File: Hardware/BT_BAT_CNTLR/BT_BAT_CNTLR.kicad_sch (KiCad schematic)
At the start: 0 parts

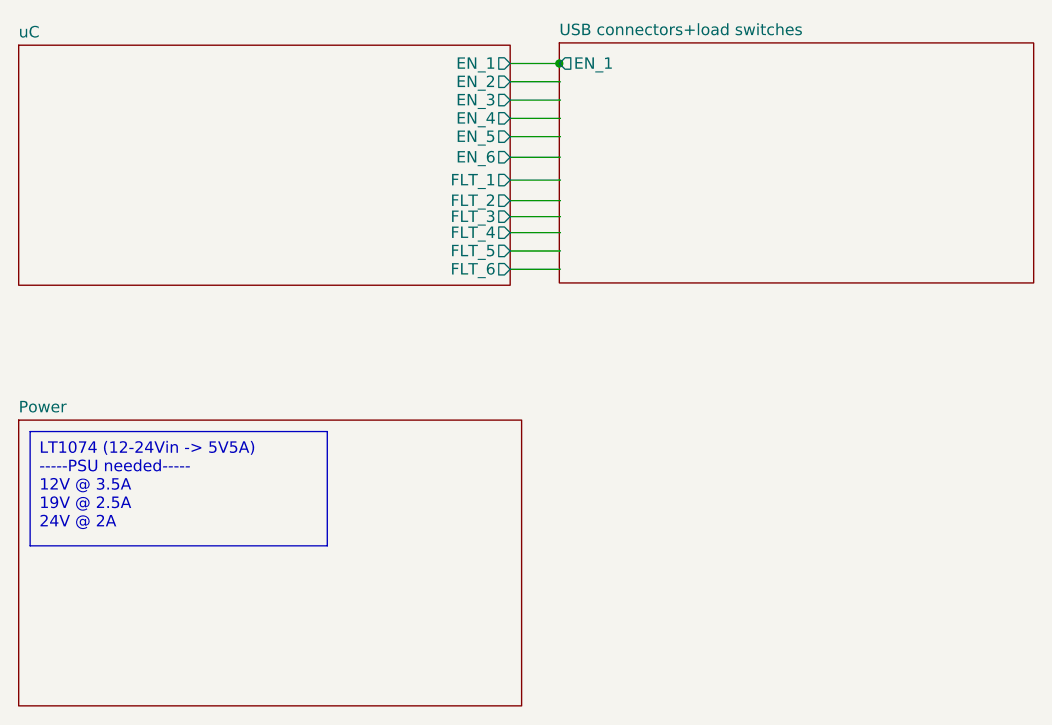
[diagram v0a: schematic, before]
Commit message: - Github Tree Cleanup - Power Routing
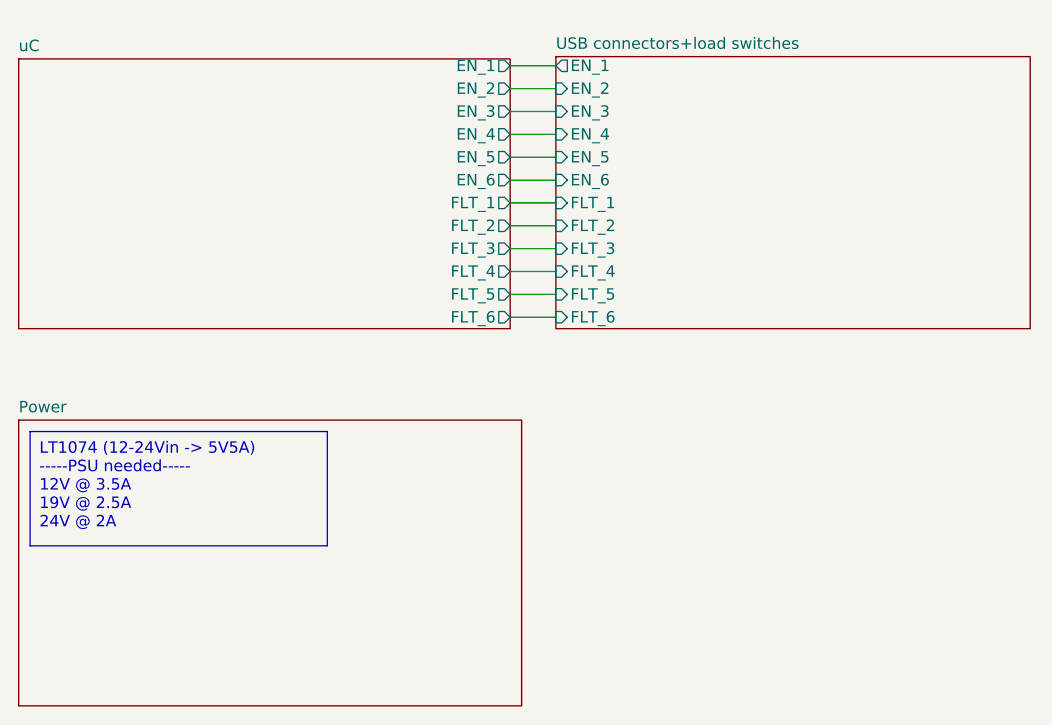
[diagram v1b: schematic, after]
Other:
- sheet USB connectors+load switches ports: added EN_2, EN_3, EN_4, EN_5, EN_6, FLT_1, FLT_2, FLT_3, FLT_4, FLT_5, FLT_6; removed none
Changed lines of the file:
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@@
 (kicad_sch (version 20230121) (generator eeschema)
   (paper "A4")
-  (junction (at 151.511 27.686) (diameter 0) (color 0 0 0 0)
-  )
-  (wire (pts (xy 146.05 38.1) (xy 151.638 38.1))
+  (wire (pts (xy 146.05 35.56) (xy 151.13 35.56))
     (stroke (width 0) (type default))
   )
-  (wire (pts (xy 146.05 29.718) (xy 151.638 29.718))
+  (wire (pts (xy 146.05 30.48) (xy 151.13 30.48))
     (stroke (width 0) (type default))
   )
-  (wire (pts (xy 146.05 27.686) (xy 151.511 27.686))
+  (wire (pts (xy 146.05 45.72) (xy 151.13 45.72))
     (stroke (width 0) (type default))
   )
-  (wire (pts (xy 146.05 33.782) (xy 151.638 33.782))
+  (wire (pts (xy 146.05 50.8) (xy 151.13 50.8))
     (stroke (width 0) (type default))
   )
-  (wire (pts (xy 146.05 46.482) (xy 151.638 46.482))
+  (wire (pts (xy 146.05 33.02) (xy 151.13 33.02))
     (stroke (width 0) (type default))
   )
-  (wire (pts (xy 146.05 42.926) (xy 151.638 42.926))
+  (wire (pts (xy 146.05 27.94) (xy 151.13 27.94))
     (stroke (width 0) (type default))
   )
-  (wire (pts (xy 146.05 50.546) (xy 151.638 50.546))
+  (wire (pts (xy 146.05 55.88) (xy 151.13 55.88))
     (stroke (width 0) (type default))
   )
-  (wire (pts (xy 146.05 48.514) (xy 151.638 48.514))
+  (wire (pts (xy 146.05 38.1) (xy 151.13 38.1))
     (stroke (width 0) (type default))
   )
-  (wire (pts (xy 146.05 40.64) (xy 151.638 40.64))
+  (wire (pts (xy 146.05 43.18) (xy 151.13 43.18))
     (stroke (width 0) (type default))
   )
-  (wire (pts (xy 146.05 35.814) (xy 151.638 35.814))
+  (wire (pts (xy 146.05 53.34) (xy 151.13 53.34))
     (stroke (width 0) (type default))
   )
-  (wire (pts (xy 146.05 44.704) (xy 151.638 44.704))
+  (wire (pts (xy 146.05 40.64) (xy 151.13 40.64))
     (stroke (width 0) (type default))
   )
-  (wire (pts (xy 151.511 27.686) (xy 151.638 27.686))
-    (stroke (width 0) (type default))
-  )
-  (wire (pts (xy 146.05 31.75) (xy 151.638 31.75))
+  (wire (pts (xy 146.05 48.26) (xy 151.13 48.26))
     (stroke (width 0) (type default))
   )
@@
     (effects (font (size 1.27 1.27)) (justify left top))
   )
-  (sheet (at 151.511 25.4) (size 52.705 26.67) (fields_autoplaced)
+  (sheet (at 151.13 26.924) (size 52.705 30.226) (fields_autoplaced)
     (stroke (width 0.1524) (type solid))
     (fill (color 0 0 0 0.0000))
-    (property "Sheetname" "USB connectors+load switches" (at 151.511 24.6884 0)
+    (property "Sheetname" "USB connectors+load switches" (at 151.13 26.2124 0)
       (effects (font (size 1.27 1.27)) (justify left bottom))
     )
-    (property "Sheetfile" "untitled.kicad_sch" (at 151.511 52.6546 0)
+    (property "Sheetfile" "untitled.kicad_sch" (at 151.13 57.7346 0)
       (effects (font (size 1.27 1.27)) (justify left top) hide)
     )
-    (pin "EN_1" output (at 151.511 27.686 180)
+    (pin "EN_1" output (at 151.13 27.94 180)
+      (effects (font (size 1.27 1.27)) (justify left))
+    )
+    (pin "FLT_1" input (at 151.13 43.18 180)
+      (effects (font (size 1.27 1.27)) (justify left))
+    )
+    (pin "FLT_2" input (at 151.13 45.72 180)
+      (effects (font (size 1.27 1.27)) (justify left))
+    )
+    (pin "EN_2" input (at 151.13 30.48 180)
+      (effects (font (size 1.27 1.27)) (justify left))
+    )
+    (pin "EN_3" input (at 151.13 33.02 180)
+      (effects (font (size 1.27 1.27)) (justify left))
+    )
+    (pin "FLT_3" input (at 151.13 48.26 180)
+      (effects (font (size 1.27 1.27)) (justify left))
+    )
+    (pin "EN_6" input (at 151.13 40.64 180)
+      (effects (font (size 1.27 1.27)) (justify left))
+    )
+    (pin "EN_5" input (at 151.13 38.1 180)
+      (effects (font (size 1.27 1.27)) (justify left))
+    )
+    (pin "EN_4" input (at 151.13 35.56 180)
+      (effects (font (size 1.27 1.27)) (justify left))
+    )
+    (pin "FLT_6" input (at 151.13 55.88 180)
+      (effects (font (size 1.27 1.27)) (justify left))
+    )
+    (pin "FLT_5" input (at 151.13 53.34 180)
+      (effects (font (size 1.27 1.27)) (justify left))
+    )
+    (pin "FLT_4" input (at 151.13 50.8 180)
       (effects (font (size 1.27 1.27)) (justify left))
     )
@@
     )
   )
-  (sheet (at 91.44 25.654) (size 54.61 26.67) (fields_autoplaced)
+  (sheet (at 91.44 27.178) (size 54.61 29.972) (fields_autoplaced)
     (stroke (width 0.1524) (type solid))
     (fill (color 0 0 0 0.0000))
-    (property "Sheetname" "uC" (at 91.44 24.9424 0)
+    (property "Sheetname" "uC" (at 91.44 26.4664 0)
       (effects (font (size 1.27 1.27)) (justify left bottom))
     )
-    (property "Sheetfile" "uC.kicad_sch" (at 91.44 52.9086 0)
+    (property "Sheetfile" "uC.kicad_sch" (at 91.44 57.7346 0)
       (effects (font (size 1.27 1.27)) (justify left top) hide)
     )
-    (pin "EN_1" output (at 146.05 27.686 0)
+    (pin "EN_1" output (at 146.05 27.94 0)
       (effects (font (size 1.27 1.27)) (justify right))
     )
-    (pin "EN_2" output (at 146.05 29.718 0)
+    (pin "EN_2" output (at 146.05 30.48 0)
       (effects (font (size 1.27 1.27)) (justify right))
     )
-    (pin "EN_3" output (at 146.05 31.75 0)
+    (pin "EN_3" output (at 146.05 33.02 0)
       (effects (font (size 1.27 1.27)) (justify right))
     )
-    (pin "EN_4" output (at 146.05 33.782 0)
+    (pin "EN_4" output (at 146.05 35.56 0)
       (effects (font (size 1.27 1.27)) (justify right))
     )
-    (pin "EN_5" output (at 146.05 35.814 0)
+    (pin "EN_5" output (at 146.05 38.1 0)
       (effects (font (size 1.27 1.27)) (justify right))
     )
-    (pin "EN_6" output (at 146.05 38.1 0)
+    (pin "EN_6" output (at 146.05 40.64 0)
       (effects (font (size 1.27 1.27)) (justify right))
     )
-    (pin "FLT_1" output (at 146.05 40.64 0)
+    (pin "FLT_1" output (at 146.05 43.18 0)
       (effects (font (size 1.27 1.27)) (justify right))
     )
-    (pin "FLT_2" output (at 146.05 42.926 0)
+    (pin "FLT_2" output (at 146.05 45.72 0)
       (effects (font (size 1.27 1.27)) (justify right))
     )
-    (pin "FLT_3" output (at 146.05 44.704 0)
+    (pin "FLT_3" output (at 146.05 48.26 0)
       (effects (font (size 1.27 1.27)) (justify right))
     )
-    (pin "FLT_6" output (at 146.05 50.546 0)
+    (pin "FLT_6" output (at 146.05 55.88 0)
       (effects (font (size 1.27 1.27)) (justify right))
     )
-    (pin "FLT_5" output (at 146.05 48.514 0)
+    (pin "FLT_5" output (at 146.05 53.34 0)
       (effects (font (size 1.27 1.27)) (justify right))
     )
-    (pin "FLT_4" output (at 146.05 46.482 0)
+    (pin "FLT_4" output (at 146.05 50.8 0)
       (effects (font (size 1.27 1.27)) (justify right))
     )
